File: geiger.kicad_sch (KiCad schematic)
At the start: 2 parts

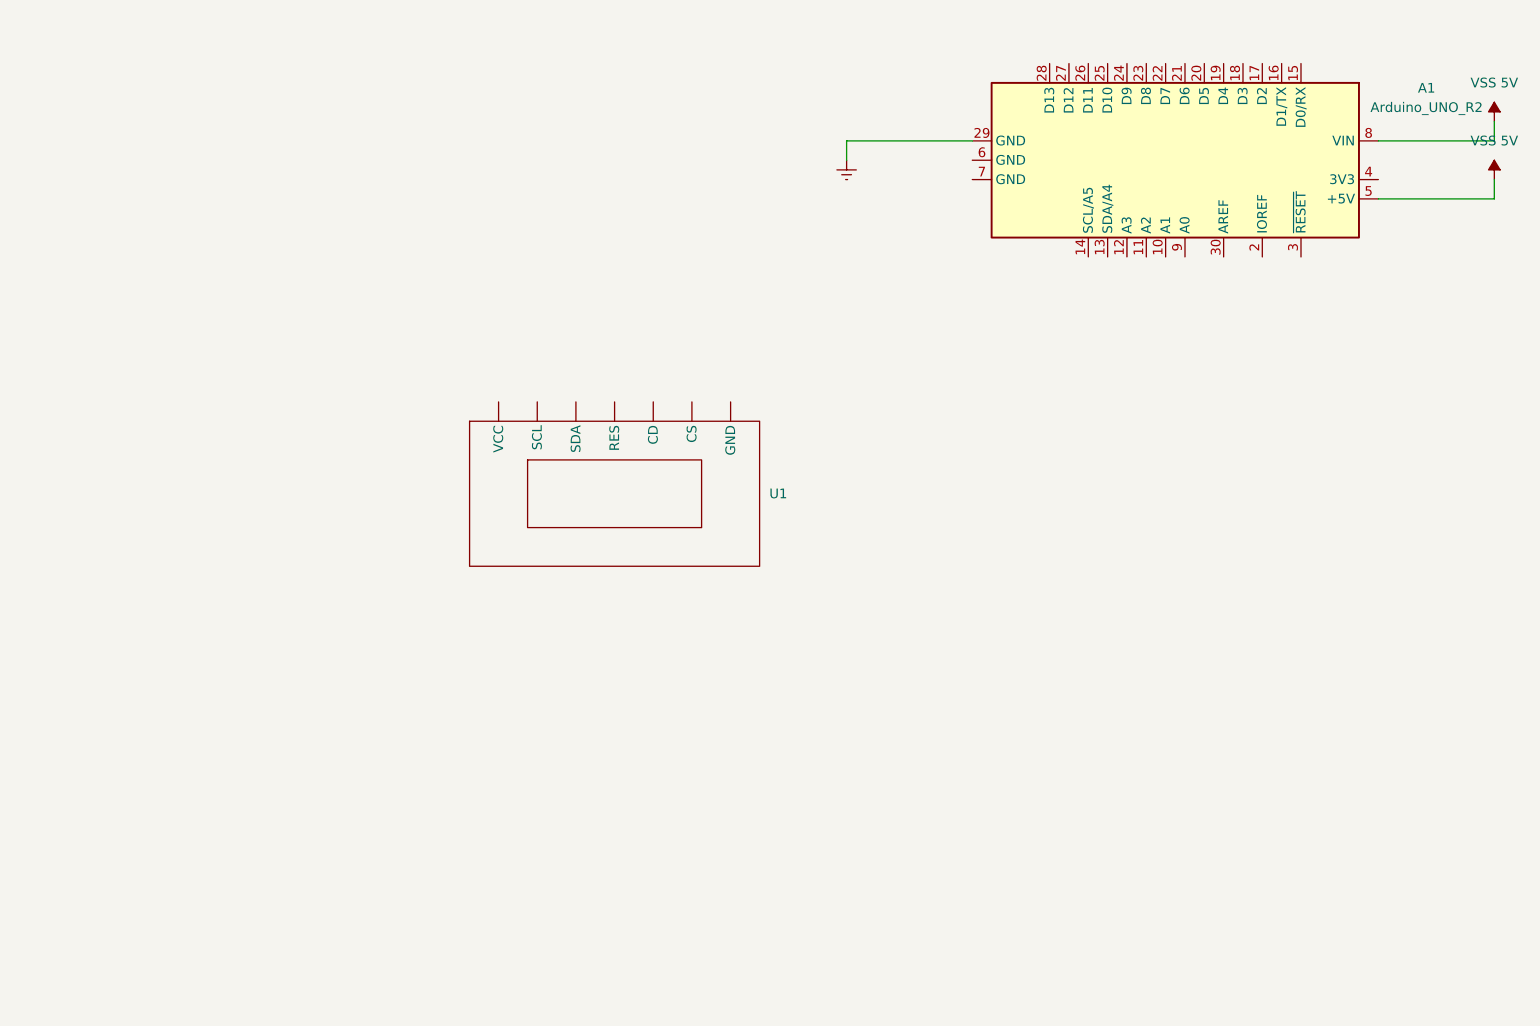
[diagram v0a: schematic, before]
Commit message: Add files via upload
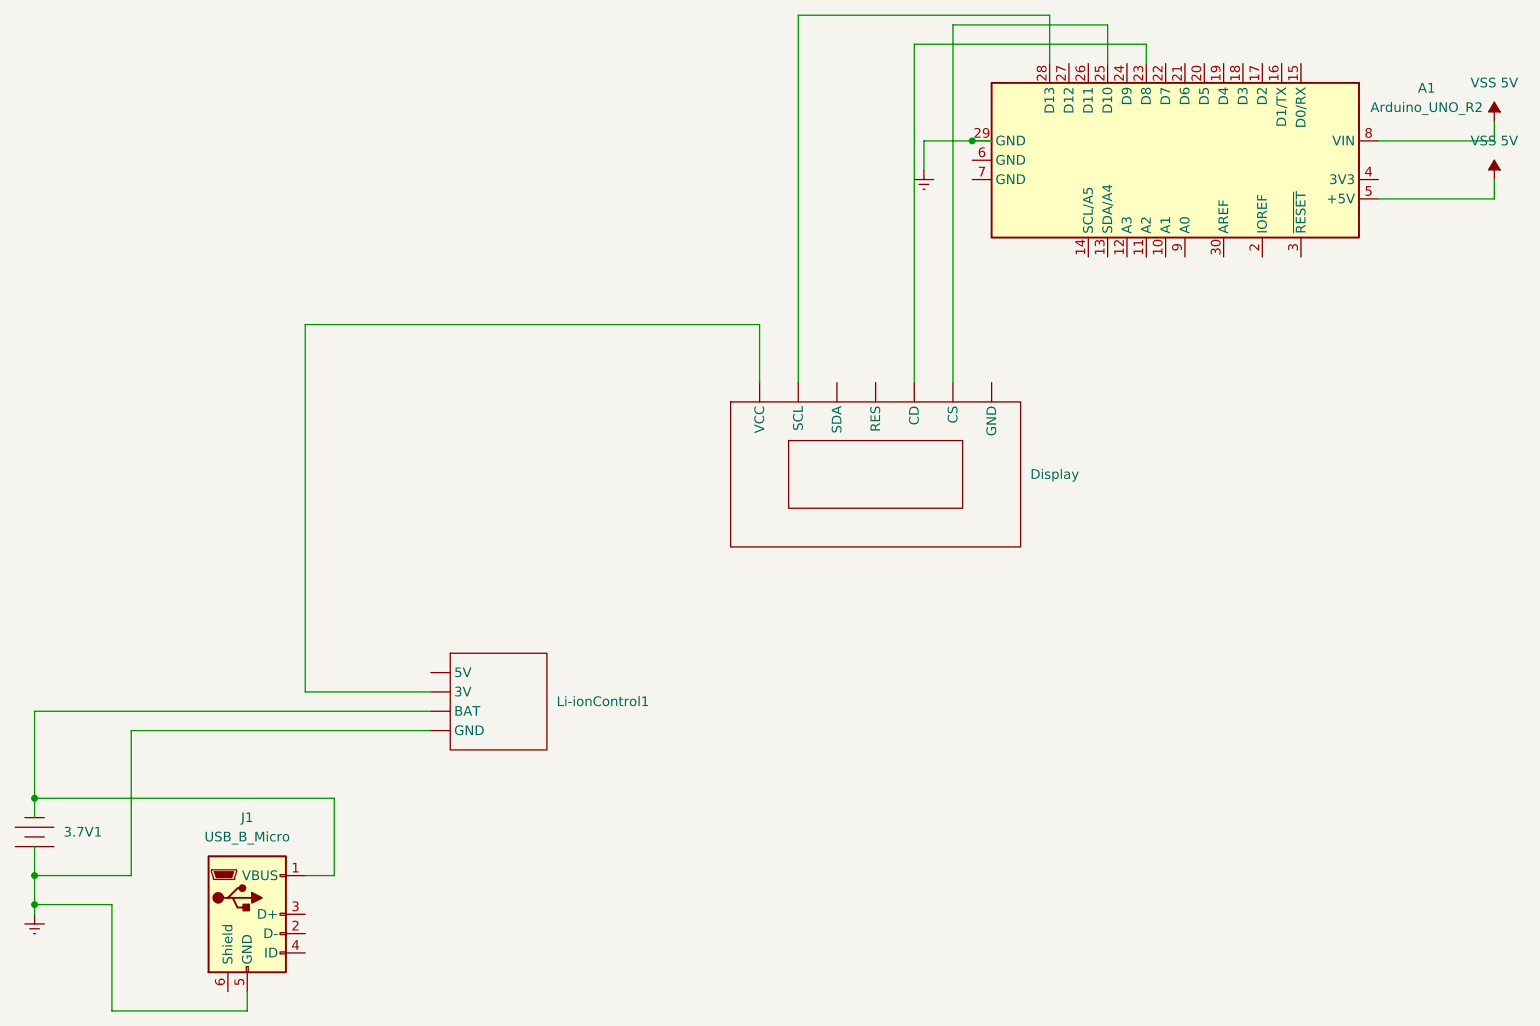
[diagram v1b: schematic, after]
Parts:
- added 3.7V1: ~, symbol geiger:3.7V_Li-Ion_Battery
- added J1: USB_B_Micro, symbol Connector:USB_B_Micro
- added Li-ionControl1: ~, symbol geiger:Li-ion_Control
- renumbered U1 to Display
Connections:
- net Earth: now also J1.5 (GND), Li-ionControl1. (GND)
- net at A1.23 (D8): now also Display. (VCC)
- net at A1.25 (D10): now also Display. (VCC)
- net at A1.28 (D13): now also Display. (VCC)
- new net: Display. (VCC), Li-ionControl1. (GND)
- new net: J1.1 (VBUS), Li-ionControl1. (GND)
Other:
- moved on the sheet: Display
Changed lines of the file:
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@@
 (kicad_sch (version 20230121) (generator eeschema)
   (paper "A4")
+  (junction (at 30.48 158.75) (diameter 0) (color 0 0 0 0)
+  )
+  (junction (at 30.48 172.72) (diameter 0) (color 0 0 0 0)
+  )
+  (junction (at 30.48 168.91) (diameter 0) (color 0 0 0 0)
+  )
+  (junction (at 153.67 72.39) (diameter 0) (color 0 0 0 0)
+  )
+  (wire (pts (xy 30.48 161.29) (xy 30.48 158.75))
+    (stroke (width 0) (type default))
+  )
+  (wire (pts (xy 30.48 158.75) (xy 69.85 158.75))
+    (stroke (width 0) (type default))
+  )
+  (wire (pts (xy 30.48 165.1) (xy 30.48 168.91))
+    (stroke (width 0) (type default))
+  )
+  (wire (pts (xy 69.85 158.75) (xy 69.85 168.91))
+    (stroke (width 0) (type default))
+  )
+  (wire (pts (xy 147.32 72.39) (xy 147.32 76.2))
+    (stroke (width 0) (type default))
+  )
+  (wire (pts (xy 176.53 62.23) (xy 176.53 59.69))
+    (stroke (width 0) (type default))
+  )
+  (wire (pts (xy 30.48 168.91) (xy 30.48 172.72))
+    (stroke (width 0) (type default))
+  )
   (wire (pts (xy 222.25 69.85) (xy 222.25 72.39))
     (stroke (width 0) (type default))
   )
+  (wire (pts (xy 125.73 96.52) (xy 125.73 104.14))
+    (stroke (width 0) (type default))
+  )
+  (wire (pts (xy 30.48 172.72) (xy 40.64 172.72))
+    (stroke (width 0) (type default))
+  )
   (wire (pts (xy 222.25 72.39) (xy 207.01 72.39))
     (stroke (width 0) (type default))
   )
-  (wire (pts (xy 137.16 72.39) (xy 137.16 74.93))
+  (wire (pts (xy 163.83 55.88) (xy 130.81 55.88))
+    (stroke (width 0) (type default))
+  )
+  (wire (pts (xy 66.04 144.78) (xy 66.04 96.52))
+    (stroke (width 0) (type default))
+  )
+  (wire (pts (xy 151.13 57.15) (xy 151.13 104.14))
+    (stroke (width 0) (type default))
+  )
+  (wire (pts (xy 69.85 168.91) (xy 66.04 168.91))
+    (stroke (width 0) (type default))
+  )
+  (wire (pts (xy 40.64 186.69) (xy 58.42 186.69))
+    (stroke (width 0) (type default))
+  )
+  (wire (pts (xy 163.83 62.23) (xy 163.83 55.88))
+    (stroke (width 0) (type default))
+  )
+  (wire (pts (xy 40.64 172.72) (xy 40.64 186.69))
+    (stroke (width 0) (type default))
+  )
+  (wire (pts (xy 30.48 147.32) (xy 82.55 147.32))
+    (stroke (width 0) (type default))
+  )
+  (wire (pts (xy 30.48 172.72) (xy 30.48 173.99))
+    (stroke (width 0) (type default))
+  )
+  (wire (pts (xy 30.48 158.75) (xy 30.48 147.32))
+    (stroke (width 0) (type default))
+  )
+  (wire (pts (xy 176.53 59.69) (xy 146.05 59.69))
+    (stroke (width 0) (type default))
+  )
+  (wire (pts (xy 171.45 62.23) (xy 171.45 57.15))
+    (stroke (width 0) (type default))
+  )
+  (wire (pts (xy 156.21 72.39) (xy 153.67 72.39))
+    (stroke (width 0) (type default))
+  )
+  (wire (pts (xy 82.55 144.78) (xy 66.04 144.78))
+    (stroke (width 0) (type default))
+  )
+  (wire (pts (xy 171.45 57.15) (xy 151.13 57.15))
     (stroke (width 0) (type default))
   )
@@
     (stroke (width 0) (type default))
   )
+  (wire (pts (xy 66.04 96.52) (xy 125.73 96.52))
+    (stroke (width 0) (type default))
+  )
+  (wire (pts (xy 146.05 59.69) (xy 146.05 104.14))
+    (stroke (width 0) (type default))
+  )
+  (wire (pts (xy 43.18 149.86) (xy 82.55 149.86))
+    (stroke (width 0) (type default))
+  )
+  (wire (pts (xy 30.48 168.91) (xy 43.18 168.91))
+    (stroke (width 0) (type default))
+  )
+  (wire (pts (xy 43.18 168.91) (xy 43.18 149.86))
+    (stroke (width 0) (type default))
+  )
+  (wire (pts (xy 58.42 186.69) (xy 58.42 184.15))
+    (stroke (width 0) (type default))
+  )
   (wire (pts (xy 222.25 80.01) (xy 207.01 80.01))
     (stroke (width 0) (type default))
   )
-  (wire (pts (xy 153.67 72.39) (xy 137.16 72.39))
-    (stroke (width 0) (type default))
+  (wire (pts (xy 147.32 72.39) (xy 153.67 72.39))
+    (stroke (width 0) (type default))
+  )
+  (wire (pts (xy 130.81 55.88) (xy 130.81 104.14))
+    (stroke (width 0) (type default))
+  )
+  (symbol (lib_id "geiger:Li-ion_Control") (at 91.44 144.78 0) (unit 1)
+    (in_bom yes) (on_board yes) (dnp no) (fields_autoplaced)
+    (property "Reference" "Li-ionControl1" (at 99.06 146.05 0)
+      (effects (font (size 1.27 1.27)) (justify left))
+    )
+    (property "Value" "~" (at 91.44 144.78 0)
+      (effects (font (size 1.27 1.27)))
+    )
+    (property "Footprint" "" (at 91.44 144.78 0)
+      (effects (font (size 1.27 1.27)) hide)
+    )
+    (property "Datasheet" "" (at 91.44 144.78 0)
+      (effects (font (size 1.27 1.27)) hide)
+    )
+    (pin "")
+    (pin "")
+    (pin "")
+    (pin "")
+    (instances
+      (project "geiger"
+        (path "/524826a5-807c-403b-9545-0bbef6be6cb1"
+          (reference "Li-ionControl1") (unit 1)
+        )
+      )
+    )
   )
   (symbol (lib_id "MCU_Module:Arduino_UNO_R2") (at 181.61 74.93 270) (unit 1)
@@
     )
   )
-  (symbol (lib_id "power:Earth") (at 137.16 74.93 0) (unit 1)
-    (in_bom yes) (on_board yes) (dnp no) (fields_autoplaced)
-    (property "Reference" "#PWR01" (at 137.16 81.28 0)
-      (effects (font (size 1.27 1.27)) hide)
-    )
-    (property "Value" "Earth" (at 137.16 78.74 0)
-      (effects (font (size 1.27 1.27)) hide)
-    )
-    (property "Footprint" "" (at 137.16 74.93 0)
-      (effects (font (size 1.27 1.27)) hide)
-    )
-    (property "Datasheet" "~" (at 137.16 74.93 0)
+  (symbol (lib_id "power:Earth") (at 30.48 173.99 0) (unit 1)
+    (in_bom yes) (on_board yes) (dnp no) (fields_autoplaced)
+    (property "Reference" "#PWR04" (at 30.48 180.34 0)
+      (effects (font (size 1.27 1.27)) hide)
+    )
+    (property "Value" "Earth" (at 30.48 177.8 0)
+      (effects (font (size 1.27 1.27)) hide)
+    )
+    (property "Footprint" "" (at 30.48 173.99 0)
+      (effects (font (size 1.27 1.27)) hide)
+    )
+    (property "Datasheet" "~" (at 30.48 173.99 0)
+      (effects (font (size 1.27 1.27)) hide)
+    )
+    (pin "1")
+    (instances
+      (project "geiger"
+        (path "/524826a5-807c-403b-9545-0bbef6be6cb1"
+          (reference "#PWR04") (unit 1)
+        )
+      )
+    )
+  )
+  (symbol (lib_id "power:Earth") (at 147.32 76.2 0) (unit 1)
+    (in_bom yes) (on_board yes) (dnp no) (fields_autoplaced)
+    (property "Reference" "#PWR01" (at 147.32 82.55 0)
+      (effects (font (size 1.27 1.27)) hide)
+    )
+    (property "Value" "Earth" (at 147.32 80.01 0)
+      (effects (font (size 1.27 1.27)) hide)
+    )
+    (property "Footprint" "" (at 147.32 76.2 0)
+      (effects (font (size 1.27 1.27)) hide)
+    )
+    (property "Datasheet" "~" (at 147.32 76.2 0)
       (effects (font (size 1.27 1.27)) hide)
     )
@@
     )
   )
-  (symbol (lib_id "Filter:OLED") (at 106.68 118.11 0) (unit 1)
-    (in_bom yes) (on_board yes) (dnp no) (fields_autoplaced)
-    (property "Reference" "U1" (at 127 118.745 0)
+  (symbol (lib_id "Filter:OLED") (at 140.97 115.57 0) (unit 1)
+    (in_bom yes) (on_board yes) (dnp no) (fields_autoplaced)
+    (property "Reference" "Display" (at 161.29 116.205 0)
       (effects (font (size 1.27 1.27)) (justify left))
     )
-    (property "Value" "~" (at 106.68 115.57 0)
-      (effects (font (size 1.27 1.27)))
-    )
-    (property "Footprint" "" (at 106.68 115.57 0)
-      (effects (font (size 1.27 1.27)) hide)
-    )
-    (property "Datasheet" "" (at 106.68 115.57 0)
-      (effects (font (size 1.27 1.27)) hide)
-    )
-    (pin "")
-    (pin "")
-    (pin "")
-    (pin "")
-    (pin "")
-    (pin "")
-    (pin "")
-    (instances
-      (project "geiger"
-        (path "/524826a5-807c-403b-9545-0bbef6be6cb1"
-          (reference "U1") (unit 1)
+    (property "Value" "~" (at 140.97 113.03 0)
+      (effects (font (size 1.27 1.27)))
+    )
+    (property "Footprint" "" (at 140.97 113.03 0)
+      (effects (font (size 1.27 1.27)) hide)
+    )
+    (property "Datasheet" "" (at 140.97 113.03 0)
+      (effects (font (size 1.27 1.27)) hide)
+    )
+    (pin "")
+    (pin "")
+    (pin "")
+    (pin "")
+    (pin "")
+    (pin "")
+    (pin "")
+    (instances
+      (project "geiger"
+        (path "/524826a5-807c-403b-9545-0bbef6be6cb1"
+          (reference "Display") (unit 1)
         )
       )
@@
         )
       )
+    )
+  )
+  (symbol (lib_id "Connector:USB_B_Micro") (at 58.42 173.99 0) (unit 1)
+    (in_bom yes) (on_board yes) (dnp no) (fields_autoplaced)
+    (property "Reference" "J1" (at 58.42 161.29 0)
+      (effects (font (size 1.27 1.27)))
+    )
+    (property "Value" "USB_B_Micro" (at 58.42 163.83 0)
+      (effects (font (size 1.27 1.27)))
+    )
+    (property "Footprint" "" (at 62.23 175.26 0)
+      (effects (font (size 1.27 1.27)) hide)
+    )
+    (property "Datasheet" "~" (at 62.23 175.26 0)
+      (effects (font (size 1.27 1.27)) hide)
+    )
+    (pin "1")
+    (pin "2")
+    (pin "3")
+    (pin "4")
+    (pin "5")
+    (pin "6")
+    (instances
+      (project "geiger"
+        (path "/524826a5-807c-403b-9545-0bbef6be6cb1"
+          (reference "J1") (unit 1)
+        )
+      )
+    )
+  )
+  (symbol (lib_id "geiger:3.7V_Li-Ion_Battery") (at 30.48 163.83 0) (unit 1)
+    (in_bom yes) (on_board yes) (dnp no) (fields_autoplaced)
+    (property "Reference" "3.7V1" (at 34.29 163.195 0)
+      (effects (font (size 1.27 1.27)) (justify left))
+    )
+    (property "Value" "~" (at 30.48 167.64 0)
+      (effects (font (size 1.27 1.27)))
+    )
+    (property "Footprint" "" (at 30.48 167.64 0)
+      (effects (font (size 1.27 1.27)) hide)
+    )
+    (property "Datasheet" "" (at 30.48 167.64 0)
+      (effects (font (size 1.27 1.27)) hide)
+    )
+    (instances
+      (project "geiger"
+        (path "/524826a5-807c-403b-9545-0bbef6be6cb1"
+          (reference "3.7V1") (unit 1)
+        )
+      )
